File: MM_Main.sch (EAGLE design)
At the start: 67 parts, among them IC1 ULN2003AD, IC2 TB6612FNG, IC4 LD117ADT50TR, Q1 TEFT4300, Q2 TEFT4300, Q3 TEFT4300, Q4 TEFT4300, Q7 8MHz, U1 STM32F405RGT6

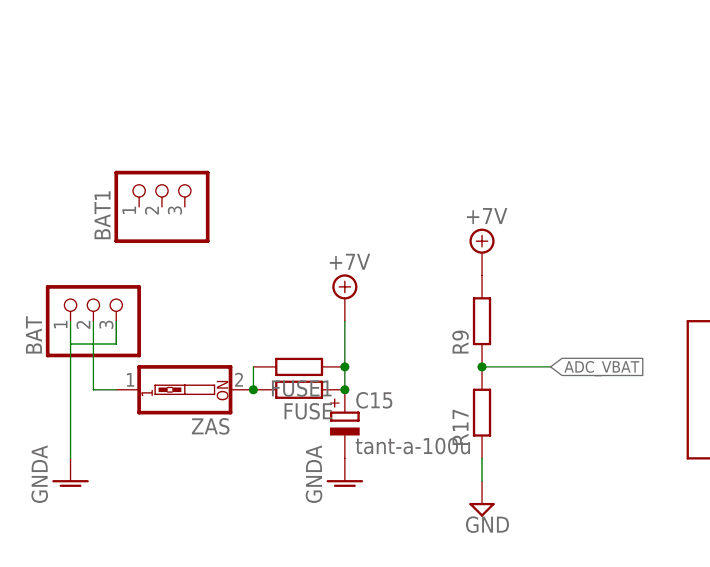
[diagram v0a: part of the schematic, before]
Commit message: aktualizacja brd
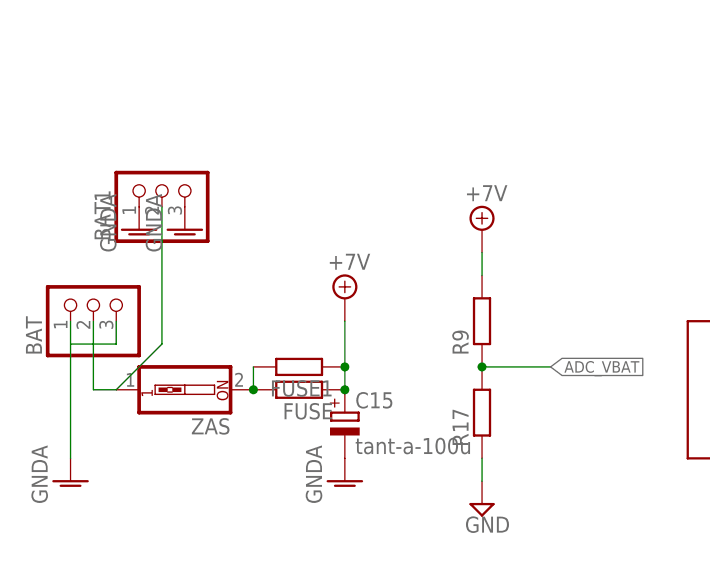
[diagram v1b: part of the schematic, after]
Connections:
- net GNDA: now also BAT1.1, BAT1.3
- net N$9: now also BAT1.2
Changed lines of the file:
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@@
 <part name="+3V5" library="supply1" deviceset="+3V3" device=""/>
 <part name="GND4" library="supply1" deviceset="GNDA" device=""/>
+<part name="GND5" library="supply1" deviceset="GNDA" device=""/>
+<part name="GND6" library="supply1" deviceset="GNDA" device=""/>
 </parts>
 <sheets>
@@
 <instance part="R9" gate="G$1" x="-106.68" y="129.54" rot="R90"/>
 <instance part="R17" gate="G$1" x="-106.68" y="119.38" rot="R90"/>
-<instance part="SUPPLY1" gate="G$1" x="-106.68" y="137.16"/>
+<instance part="SUPPLY1" gate="G$1" x="-106.68" y="139.7"/>
 <instance part="R18" gate="G$1" x="269.24" y="12.7"/>
 <instance part="R19" gate="G$1" x="274.32" y="7.62" rot="R90"/>
@@
 </instance>
 <instance part="GND4" gate="1" x="-152.4" y="111.76"/>
+<instance part="GND5" gate="1" x="-144.78" y="139.7"/>
+<instance part="GND6" gate="1" x="-139.7" y="139.7"/>
 </instances>
 <busses>
@@
 <pinref part="GND4" gate="1" pin="GNDA"/>
 </segment>
+<segment>
+<pinref part="BAT1" gate="A" pin="1"/>
+<pinref part="GND5" gate="1" pin="GNDA"/>
+</segment>
+<segment>
+<pinref part="BAT1" gate="A" pin="3"/>
+<pinref part="GND6" gate="1" pin="GNDA"/>
+</segment>
 </net>
 <net name="+3V3" class="0">
@@
 <pinref part="R9" gate="G$1" pin="2"/>
 <pinref part="SUPPLY1" gate="G$1" pin="+7V"/>
+<wire x1="-106.68" y1="137.16" x2="-106.68" y2="134.62" width="0.1524" layer="91"/>
 </segment>
 <segment>
@@
 <pinref part="ZAS" gate="G$1" pin="1"/>
 <wire x1="-149.86" y1="121.92" x2="-147.32" y2="121.92" width="0.1524" layer="91"/>
-</segment>
-</net>
+<pinref part="BAT1" gate="A" pin="2"/>
+<wire x1="-142.24" y1="142.24" x2="-142.24" y2="127" width="0.1524" layer="91"/>
+<wire x1="-142.24" y1="127" x2="-147.32" y2="121.92" width="0.1524" layer="91"/>
+</segment>
+</net>
